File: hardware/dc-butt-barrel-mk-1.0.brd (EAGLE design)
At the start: 22.9 x 17.8 mm, 13 parts, among them U1_ ROTARY_ENCODER_SWITCH, U2 Tiny85

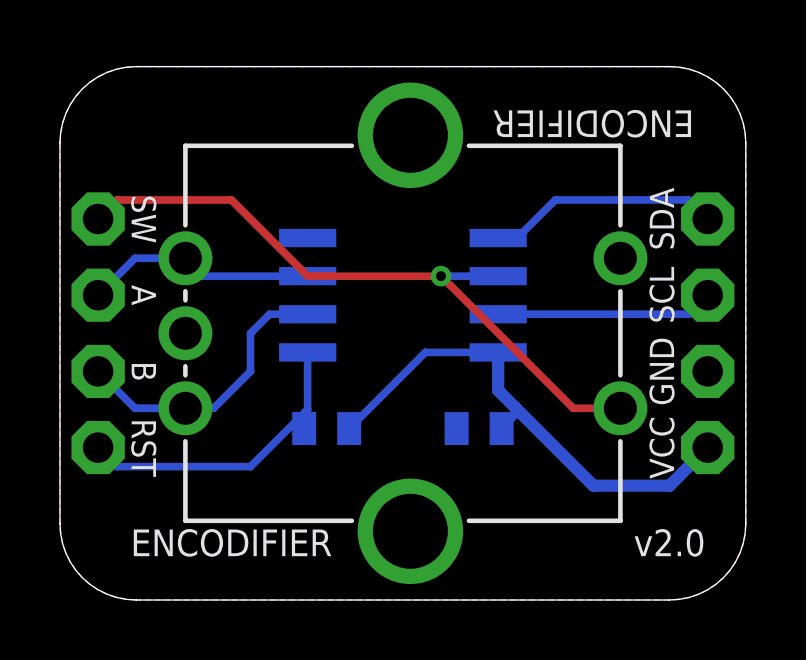
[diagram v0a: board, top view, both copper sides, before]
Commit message: have some boards, dawg
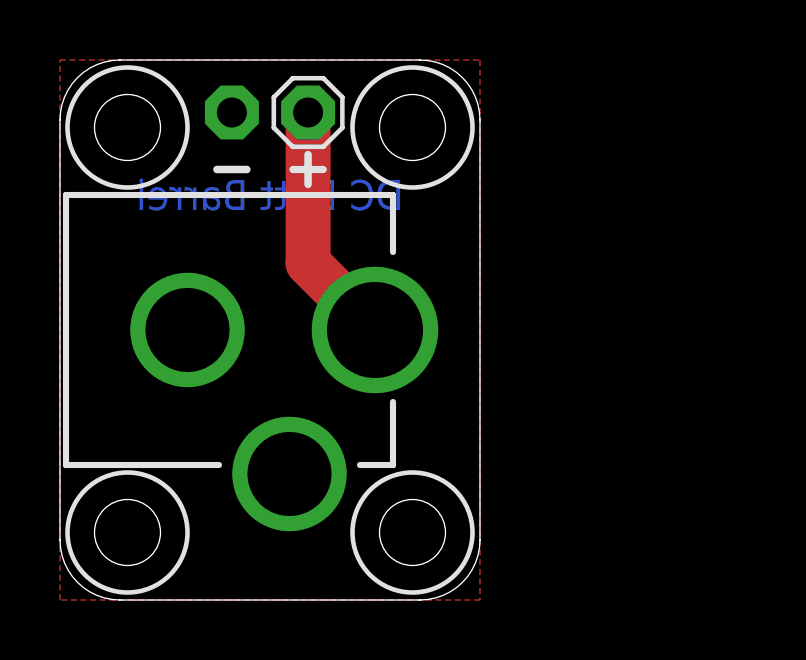
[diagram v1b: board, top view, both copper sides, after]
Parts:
- removed A, B, GND, RST, SCL, SDA, SW, VCC: M01PTH-1MM, a_parts:1X01-1MM-NS
- removed C1: 100n, a_parts:C0603-TIGHTER
- removed R1: 10k, a_parts:R0603-TIGHTER
- removed U1_: ROTARY_ENCODER_SWITCH, a_parts:ROTARY_ENCODER_SWITCH
- removed U2: Tiny85, a_parts:SO08-EIAJ
- added JP1: M02PTH-CENTERED-R+, a_parts:1X02-CENTER-R+
- added PWR1: DCBARRELPTH, a_parts:DCJACK_2MM_PTH
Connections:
- removed net A: A.1, U1_.A, U2.3
- removed net B: B.1, U1_.B, U2.2
- removed net MOSI/SDA: SDA.1, U2.5
- removed net RST: R1.1, RST.1, U2.1
- removed net SCK/SCL: SCL.1, U2.7
- removed net SW: SW.1, U1_.SW1, U2.6
- removed net VCC: C1.1, R1.2, U2.8, VCC.1
- new net VIN: JP1.2, PWR1.PWR
- net GND: now also JP1.1, PWR1.BRK, PWR1.GND; no longer C1.2, GND.1, U1_.C, U1_.SW2, U2.4
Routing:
- net SW: track 22.5 -> 0.00 mm, vias 1 -> 0
- net VCC: track 17.0 -> 0.00 mm
- net RST: track 10.5 -> 0.00 mm
- net B: track 9.54 -> 0.00 mm
- net VIN: track 0.00 -> 8.17 mm
- net MOSI/SDA: track 7.77 -> 0.00 mm
- net A: track 7.74 -> 0.00 mm
- net SCK/SCL: track 7.25 -> 0.00 mm
- removed copper zone on layer 16, net GND
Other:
- board size 22.9 x 17.8 mm -> 14 x 18 mm
- board text added: "DC Butt Barrel"
- board text removed: "A"
- board text removed: "B"
- board text removed: "C"
- board text removed: "COM"
- board text removed: "ENCODIFIER"
- board text removed: "SW"
